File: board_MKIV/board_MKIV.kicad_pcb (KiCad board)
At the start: 2 copper layers, 100 x 120 mm, 43 parts, among them J1 1757242, J2 jst-power, J3 JST -SM, J5 1770979, J6 20_pin_90, J7 20-pin-straight, U1 ESP32-DEVKITC-32D, U2 LTV-846S, U3 TLV272CDR, U4 BAT46W, U5 BA&, U6 SH-7070TB

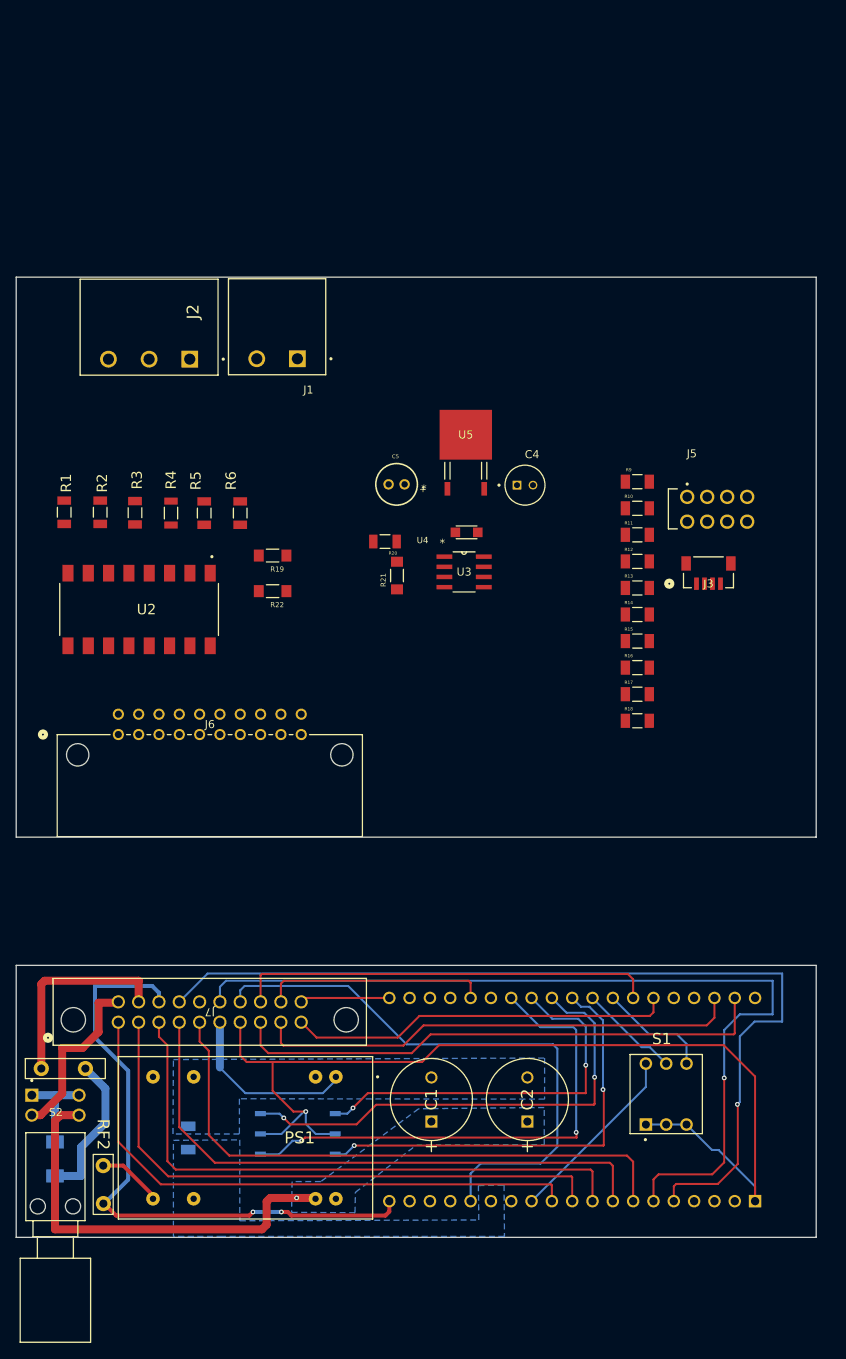
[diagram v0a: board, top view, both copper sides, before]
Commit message: update
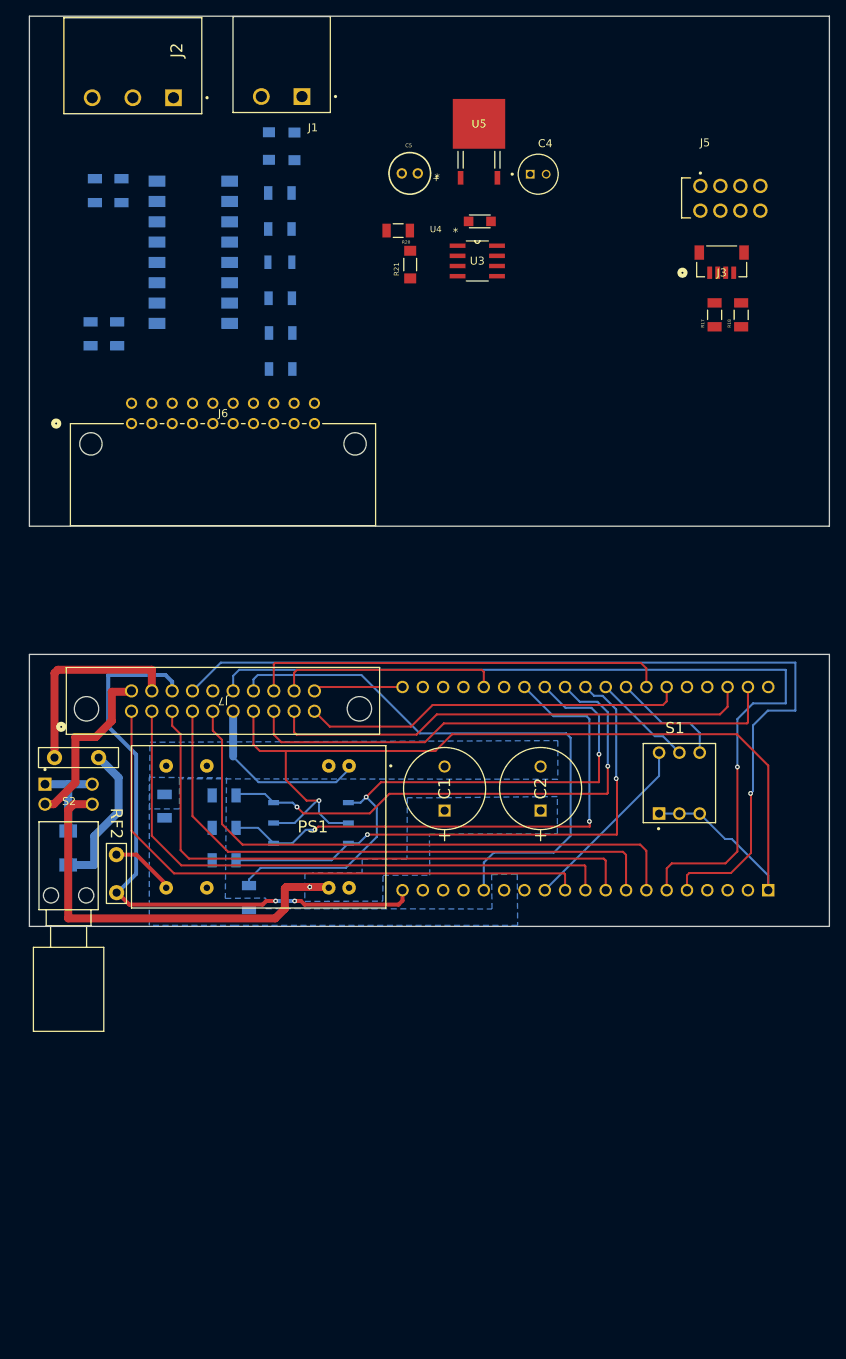
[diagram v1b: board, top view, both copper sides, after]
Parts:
- R1, R10, R11, R12, R13, R14, R15, R16, R19, R2, R22, R3, R4, R5, R6, R9, U2: moved to B.Cu
- moved R10 78.6 mm to (57.3, 57.4), turned to 90 degrees
- moved R9 74.0 mm to (60.6, 57.4), turned to 90 degrees
- moved R12 74.0 mm to (56.8, 75.3), turned to 90 degrees
- moved R11 69.7 mm to (60.1, 75.3), turned to 90 degrees
- moved R14 60.1 mm to (73.4, 141.1), turned to 180 degrees
- moved R15 58.2 mm to (76.5, 145.8), turned to -90 degrees
- moved R13 57.8 mm to (73.4, 133.0), turned to 180 degrees
- moved R22 55.6 mm to (79.0, 51.9), turned to -90 degrees
- moved R16 55.4 mm to (73.4, 137.1), turned to 180 degrees
- moved R18 52.4 mm to (138.1, 73.0), turned to 90 degrees
- moved R19 51.2 mm to (82.2, 51.9), turned to -90 degrees
- moved R17 48.4 mm to (134.8, 73.0), turned to 90 degrees
- moved U2 45.2 mm to (69.6, 65.1), turned to 180 degrees
- moved C3 41.6 mm to (66.0, 134.4)
- moved R6 40.3 mm to (80.4, 57.7), turned to 180 degrees
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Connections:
- R10 pad 1: GPIO_33_ -> GPIO_33
- R11 pad 1: GPIO_26_ -> GPIO_26
- R12 pad 1: GPIO_25_ -> GPIO_25
- R9 pad 1: GPIO_32_ -> GPIO_32
- U2 pad 10: GPIO_32_ -> GPIO_32
- U2 pad 12: GPIO_33_ -> GPIO_33
- U2 pad 14: GPIO_25_ -> GPIO_25
- U2 pad 16: GPIO_26_ -> GPIO_26
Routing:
- net GPIO_16: track 49.5 -> 74.0 mm
- net GPIO_5: track 55.3 -> 70.3 mm
- net GPIO_4: track 64.2 -> 69.8 mm
- net GPIO_17: track 60.7 -> 66.0 mm
- net +VOUT_esp_signal: track 77.8 -> 77.3 mm
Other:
- board size 100 x 120 mm -> 100 x 113.8 mm
